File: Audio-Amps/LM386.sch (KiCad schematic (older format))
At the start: 6 parts, among them U1 LM386

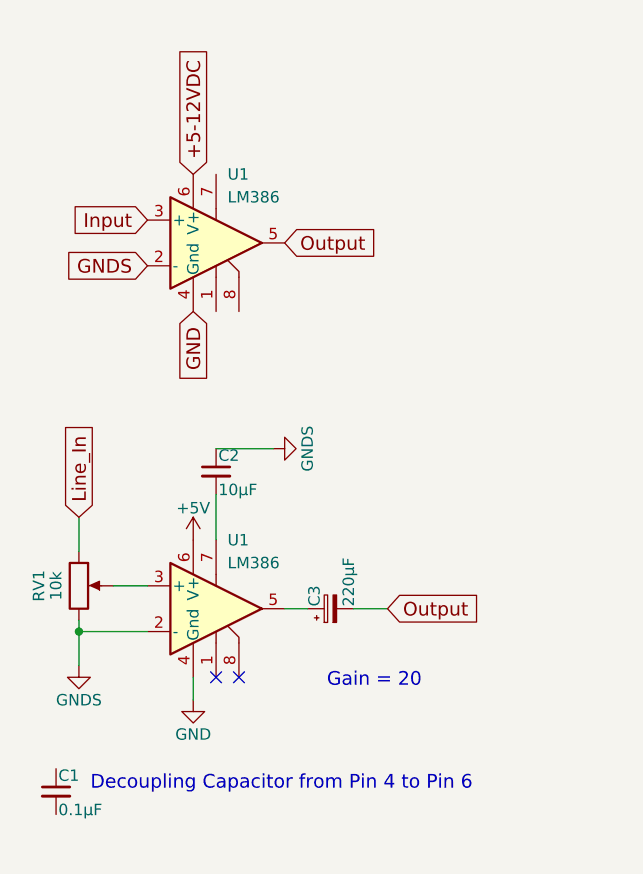
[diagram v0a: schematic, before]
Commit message: WIP
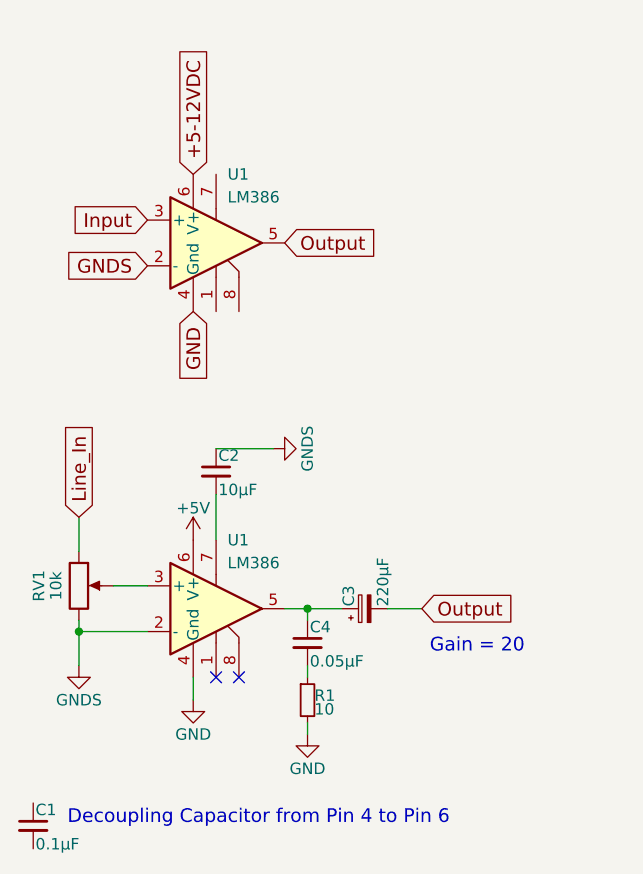
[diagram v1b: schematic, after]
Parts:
- added C4: 0.05µF, symbol C_Small
- added R1: 10, symbol R_Small
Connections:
- net GND: now also R1.2
- net at C3.1, U1.5: now also C4.1
- new net: C4.2, R1.1
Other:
- moved on the sheet: C1, C3
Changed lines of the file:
@@
 $EndComp
 Wire Wire Line
-	4750 3550 4750 3750
+	4750 3550 4750 3600
+Wire Wire Line
+	4750 3600 4750 3750
 Wire Wire Line
 	5050 3600 4750 3600
@@
 L CP_Small C3
 U 1 1 59F13A30
-P 5850 3500
-F 0 "C3" H 5860 3570 50  0000 L CNN
-F 1 "220µF" H 5860 3420 50  0000 L CNN
-F 2 "" H 5850 3500 50  0001 C CNN
-F 3 "" H 5850 3500 50  0001 C CNN
-	1    5850 3500
+P 6000 3500
+F 0 "C3" H 6010 3570 50  0000 L CNN
+F 1 "220µF" H 6010 3420 50  0000 L CNN
+F 2 "" H 6000 3500 50  0001 C CNN
+F 3 "" H 6000 3500 50  0001 C CNN
+	1    6000 3500
 	0    -1   -1   0
 $EndComp
 Wire Wire Line
-	5750 3500 5650 3500
+	5650 3500 5750 3500
+Wire Wire Line
+	5750 3500 5900 3500
 $Comp
 L GND #PWR3
@@
 NoConn ~ 5350 3800
 NoConn ~ 5450 3800
-Text GLabel 6100 3500 2    60   Input ~ 0
+Text GLabel 6250 3500 2    60   Input ~ 0
 Output
 Wire Wire Line
-	6100 3500 5950 3500
-Text Notes 6250 3850 2    60   ~ 0
+	6250 3500 6100 3500
+Text Notes 6700 3700 2    60   ~ 0
 Gain = 20
 $Comp
 L C_Small C1
 U 1 1 59F13B74
-P 4650 4300
-F 0 "C1" H 4660 4370 50  0000 L CNN
-F 1 "0.1µF" H 4660 4220 50  0000 L CNN
-F 2 "" H 4650 4300 50  0001 C CNN
-F 3 "" H 4650 4300 50  0001 C CNN
-	1    4650 4300
+P 4550 4450
+F 0 "C1" H 4560 4520 50  0000 L CNN
+F 1 "0.1µF" H 4560 4370 50  0000 L CNN
+F 2 "" H 4550 4450 50  0001 C CNN
+F 3 "" H 4550 4450 50  0001 C CNN
+	1    4550 4450
 	1    0    0    -1
 $EndComp
-Text Notes 4800 4300 0    60   ~ 0
+Text Notes 4700 4450 0    60   ~ 0
 Decoupling Capacitor from Pin 4 to Pin 6
+$Comp
+L C_Small C4
+U 1 1 59F13DAD
+P 5750 3650
+F 0 "C4" H 5760 3720 50  0000 L CNN
+F 1 "0.05µF" H 5760 3570 50  0000 L CNN
+F 2 "" H 5750 3650 50  0001 C CNN
+F 3 "" H 5750 3650 50  0001 C CNN
+	1    5750 3650
+	1    0    0    -1
+$EndComp
+Wire Wire Line
+	5750 3500 5750 3550
+Connection ~ 5750 3500
+$Comp
+L R_Small R1
+U 1 1 59F13FFF
+P 5750 3900
+F 0 "R1" H 5780 3920 50  0000 L CNN
+F 1 "10" H 5780 3860 50  0000 L CNN
+F 2 "" H 5750 3900 50  0001 C CNN
+F 3 "" H 5750 3900 50  0001 C CNN
+	1    5750 3900
+	1    0    0    -1
+$EndComp
+Wire Wire Line
+	5750 3750 5750 3800
+Wire Wire Line
+	5750 4000 5750 4050
+$Comp
+L GND #PWR?
+U 1 1 59F14169
+P 5750 4050
+F 0 "#PWR?" H 5750 3800 50  0001 C CNN
+F 1 "GND" H 5750 3900 50  0000 C CNN
+F 2 "" H 5750 4050 50  0001 C CNN
+F 3 "" H 5750 4050 50  0001 C CNN
+	1    5750 4050
+	1    0    0    -1
+$EndComp
 $EndSCHEMATC
